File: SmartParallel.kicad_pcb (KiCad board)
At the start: 2 copper layers, 93.7 x 60.5 mm, 50 parts, among them IC1 S74HC595, J1 DB25, P1 SERIAL_PORT, P2 PWR_IN, P3 PWR_OUT, P4 PWR_OUT, P5 I2C_DISPLAY, P6 RESET, SW2 SW_RST, U1 328PB, U2 74HC541, U3 74HC14MS, Y1 16MHz

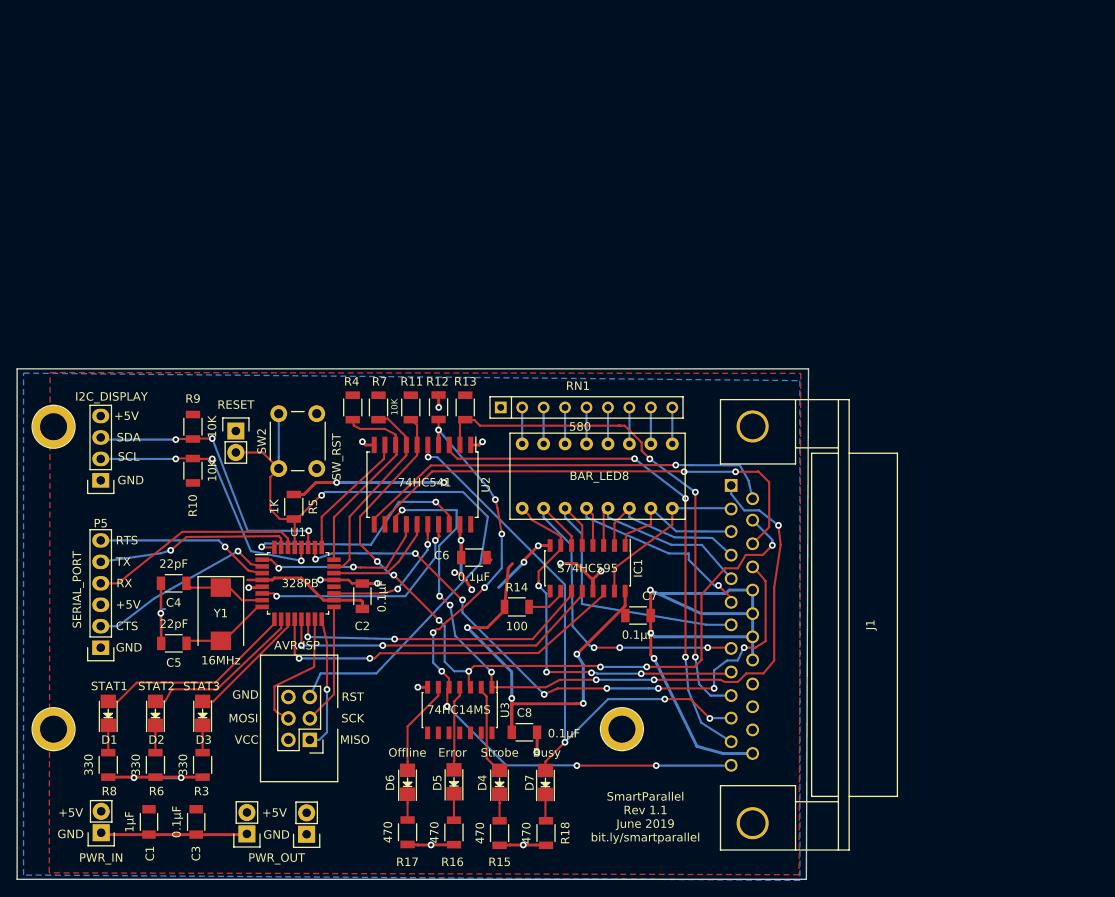
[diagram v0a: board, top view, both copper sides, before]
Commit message: Misc tweaks
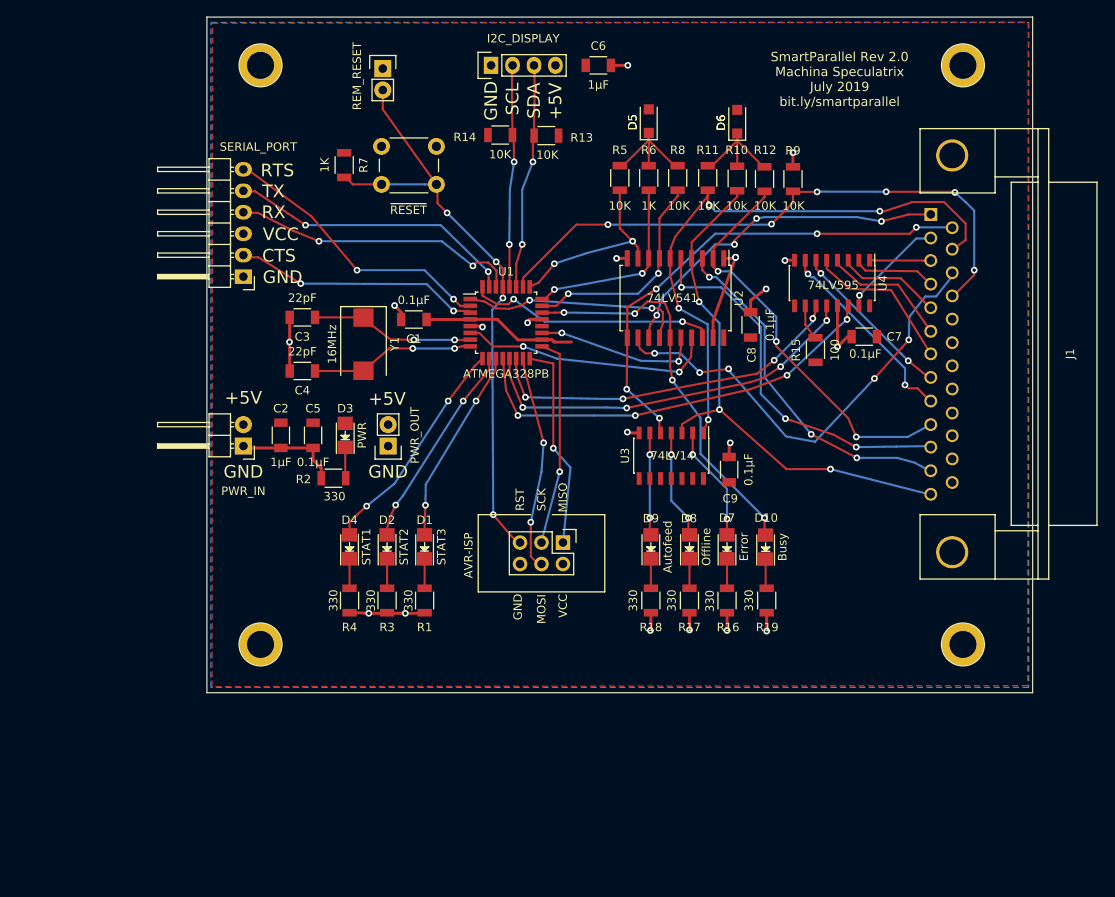
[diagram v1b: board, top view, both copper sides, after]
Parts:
- removed IC1: S74HC595, Housings_SOIC:SOIC-16_3.9x9.9mm_Pitch1.27mm
- removed LED1: BAR_LED8, Speculatrix_general:8-bar LED
- removed P6: RESET, Pin_Headers:Pin_Header_Straight_1x02
- removed the REF** at (172.0, 109.2)
- removed the REF** at (104.6, 109.2)
- removed the REF** at (104.6, 73.4)
- removed RN1: 580, Resistors_ThroughHole:Resistor_Array_SIP8
- removed SW2: SW_RST, Buttons_Switches_ThroughHole:SW_PUSH_6mm
- added C9: 0.1µF, Capacitors_SMD:C_1206, F.Cu at (184.7, 78.5)
- added D10: Busy, LEDs:LED_1206, F.Cu at (189.0, 87.7)
- added D8: Offline, LEDs:LED_1206, F.Cu at (180.0, 87.6)
- added D9: Autofeed, LEDs:LED_1206, F.Cu at (175.4, 87.6)
- added R1: 330, Resistors_SMD:R_1206, F.Cu at (148.6, 94.0)
- added R19: 330, Resistors_SMD:R_1206, F.Cu at (189.1, 94.0)
- added R2: 330, Resistors_SMD:R_1206, F.Cu at (137.8, 79.5)
- added REF**: M3, Speculatrix_general:Mounting_hole_M3, F.Cu at (212.3, 99.2)
- added REF**: M3, Speculatrix_general:Mounting_hole_M3, F.Cu at (129.2, 99.2)
- added REF**: M3, Speculatrix_general:Mounting_hole_M3, F.Cu at (129.2, 30.6)
- added REF**: M3, Speculatrix_general:Mounting_hole_M3, F.Cu at (212.3, 30.6)
- added SW1: ~RESET, Buttons_Switches_ThroughHole:SW_PUSH_6mm, F.Cu at (150.0, 44.7)
- added U4: 74LV595, Housings_SOIC:SOIC-16_3.9x9.9mm_Pitch1.27mm, F.Cu at (196.8, 56.4)
- C1: value 1µF -> 0.1µF
- C2, C6: value 0.1µF -> 1µF
- C3: value 0.1µF -> 22pF
- C5: value 22pF -> 0.1µF
- D1: value STAT1 -> STAT3
- D3: value STAT3 -> PWR
- D4: value Strobe -> STAT1
- D5: value Error -> D; footprint LEDs:LED_1206 -> Speculatrix_general:Diode_SOD-123F-S-FLAT
- D6: value Offline -> D; footprint LEDs:LED_1206 -> Speculatrix_general:Diode_SOD-123F-S-FLAT
- D7: value Busy -> Error
- P1: footprint Pin_Headers:Pin_Header_Straight_1x06 -> Pin_Headers:Pin_Header_Angled_1x06
- P2: footprint Pin_Headers:Pin_Header_Straight_1x02 -> Pin_Headers:Pin_Header_Angled_1x02
- P4: value PWR_OUT -> I2C_DISPLAY; footprint Pin_Headers:Pin_Header_Straight_1x02 -> Pin_Headers:Pin_Header_Straight_1x04
- P5: value I2C_DISPLAY -> REM_RESET; footprint Pin_Headers:Pin_Header_Straight_1x04 -> Pin_Headers:Pin_Header_Straight_1x02
- R10: value 10K -> 10k
- R11: value 10k -> 10K
- R14: value 100 -> 10K
- R15: value 470 -> 100
- R16, R17, R18: value 470 -> 330
- R4: value 10K -> 330
- R5: value 1K -> 10K
- R6: value 330 -> 1K
- R7: value 10K -> 1K
- R8: value 330 -> 10K
- U1: value 328PB -> ATMEGA328PB
- U2: value 74HC541 -> 74LV541
- U3: value 74HC14MS -> 74LV14
- moved R8 96.8 mm to (178.6, 43.9)
- moved P4 93.6 mm to (156.5, 30.6), turned to 90 degrees
- moved R6 90.8 mm to (175.1, 43.9)
- moved D6 87.4 mm to (185.6, 37.3)
- moved D5 81.6 mm to (175.1, 37.2)
- moved R9 76.9 mm to (192.2, 44.1), turned to 90 degrees
- moved R10 73.2 mm to (185.6, 44.0), turned to 270 degrees
- moved R15 68.4 mm to (194.9, 64.3), turned to 90 degrees
- moved C1 67.3 mm to (147.3, 60.7), turned to 180 degrees
- moved C3 61.1 mm to (134.1, 60.5), turned to 180 degrees
- moved C6 60.1 mm to (169.2, 30.6), turned to 0 degrees
- moved P5 59.1 mm to (143.6, 31.0), turned to 0 degrees
- moved R14 55.9 mm to (157.5, 38.9)
- moved C8 55.2 mm to (187.2, 61.3), turned to 90 degrees
- moved R5 54.8 mm to (171.7, 43.9)
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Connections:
- net Ack_buf renamed ~Ack_buf
- net Err_buf renamed ~Err_buf
- net Init_buf renamed ~Init_buf
- C3 pad 1: VCC -> /XTAL1
- C4 pad 1: /XTAL1 -> /XTAL2
- C5 pad 1: /XTAL2 -> VCC
- D1 pad 2: Stat1 -> Stat3
- D3 pad 2: Stat3 -> VCC
- D4 pad 2: Net-(D4-Pad2) -> Stat1
- D5 pad 2: Net-(D5-Pad2) -> VCC
- D6 pad 2: Net-(D6-Pad2) -> VCC
- D7 pad 2: Busy -> Net-(D7-Pad2)
- J1 pad 1: Strobe_buf -> ~Strobe_buf
- J1 pad 14: LF_buf -> ~Autofeed_buf
- J1 pad 17: ~SelIn -> SelIn
- P4 pad 2: VCC -> SCL
- P5 pad 2: SCL -> ~RESET
- R10 pad 1: VCC -> Net-(D6-Pad1)
- R10 pad 2: SCL -> SEL
- R11 pad 1: SEL -> Net-(D6-Pad1)
- R11 pad 2: GND -> ~Error
- R12 pad 1: VCC -> Net-(D6-Pad1)
- R12 pad 2: ~Error -> ~ACK
- R13 pad 2: ~ACK -> SDA
- R14 pad 2: Net-(IC1-Pad10) -> SCL
- R15 pad 1: Net-(D4-Pad1) -> VCC
- R15 pad 2: GND -> Net-(R15-Pad2)
- R16 pad 1: Net-(D5-Pad1) -> Net-(D7-Pad1)
- R17 pad 1: Net-(D6-Pad1) -> Net-(D8-Pad1)
- R18 pad 1: Net-(D7-Pad1) -> Net-(D9-Pad1)
- R3 pad 1: Net-(D3-Pad1) -> Net-(D2-Pad1)
- R4 pad 1: VCC -> Net-(D4-Pad1)
- R4 pad 2: ~Init -> GND
- R5 pad 1: VCC -> Net-(D5-Pad1)
- R5 pad 2: ~RESET -> ~Autofeed
- R6 pad 1: Net-(D2-Pad1) -> Net-(D5-Pad1)
- R6 pad 2: GND -> ~Init
- R7 pad 2: ~Strobe -> ~RESET
- R8 pad 1: Net-(D1-Pad1) -> Net-(D5-Pad1)
- R8 pad 2: GND -> ~Strobe
- R9 pad 1: VCC -> SelIn
- R9 pad 2: SDA -> GND
- U1 pad 2: CTS -> RTS
- U1 pad 25: LF -> ~Autofeed
- U1 pad 26: ~SelIn -> SelIn
- U1 pad 3: RTS -> CTS
- U2 pad 11: LF_buf -> ~Autofeed_buf
- U2 pad 13: Strobe_buf -> ~Strobe_buf
- U2 pad 9: LF -> ~Autofeed
- U3 pad 1: Strobe_buf -> ~Error
- U3 pad 2: Net-(D4-Pad2) -> Net-(D7-Pad2)
- U3 pad 3: ~Error -> SEL
- U3 pad 4: Net-(D5-Pad2) -> Net-(D8-Pad2)
- U3 pad 5: SEL -> ~Autofeed_buf
- U3 pad 6: Net-(D6-Pad2) -> Net-(D9-Pad2)
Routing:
- net GND: track 170.1 -> 72.4 mm, vias 23 -> 20
- net Strobe_buf: track 91.8 -> 0.00 mm, vias 7 -> 0
- net ~SelIn: track 75.9 -> 0.00 mm, vias 8 -> 0
- net SelIn: track 0.00 -> 71.8 mm, vias 0 -> 6
- net VCC: track 88.9 -> 17.8 mm, vias 6 -> 0
- net ~Autofeed_buf: track 0.00 -> 58.5 mm, vias 0 -> 5
- net LF_buf: track 50.8 -> 0.00 mm, vias 1 -> 0
- net ~Strobe_buf: track 0.00 -> 40.7 mm, vias 0 -> 4
- net Busy_buf: track 13.3 -> 46.8 mm, vias 0 -> 4
- net Busy: track 69.9 -> 44.7 mm, vias 4 -> 3
- net ~Error: track 92.4 -> 69.9 mm, vias 7 -> 4
- net ~Autofeed: track 0.00 -> 22.2 mm, vias 0 -> 2
- net D7: track 45.4 -> 23.6 mm, vias 4 -> 2
- net D6: track 41.0 -> 19.6 mm, vias 3 -> 2
- net PE: track 61.7 -> 41.7 mm
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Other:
- board size 93.7 x 60.5 mm -> 97.8 x 80 mm
- board text added: "SmartParallel Rev 2.0 Machina Speculatrix July 2019 bit.ly/smartparallel"
- board text added: "VCC"
- board text removed: "SmartParallel Rev 1.1 June 2019 bit.ly/smartparallel"
